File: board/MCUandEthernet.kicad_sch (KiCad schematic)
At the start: 3 parts, among them J1 RJ45_LED_Shielded, U15 Teensy4.1_DEV-16771

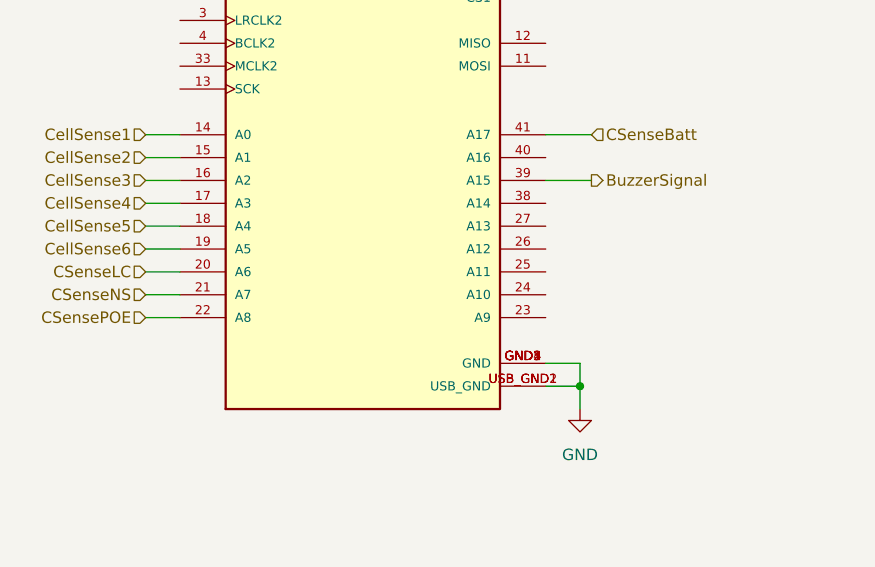
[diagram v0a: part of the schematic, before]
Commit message: Replaced Current sensors and made aux current sensor
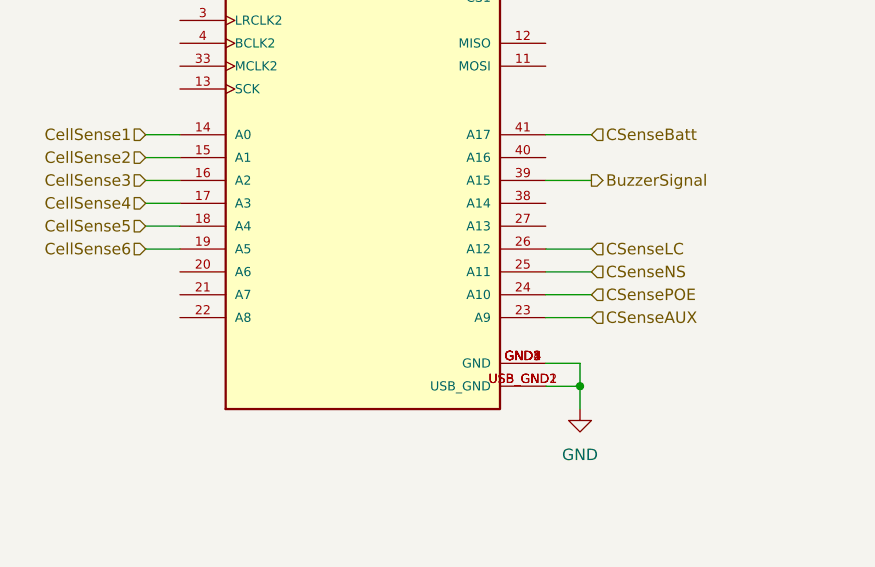
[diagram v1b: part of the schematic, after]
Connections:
- net CSenseLC: now also U15.26 (A12); no longer U15.20 (A6)
- net CSenseNS: now also U15.25 (A11); no longer U15.21 (A7)
- net CSensePOE: now also U15.24 (A10); no longer U15.22 (A8)
- net CSenseAUX: now reaches U15.23 (A9)
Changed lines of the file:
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@@
-	(wire
-		(pts
-			(xy 24.13 134.62) (xy 27.94 134.62)
-		)
-		(stroke
-			(width 0)
-			(type default)
-		)
-	)
 	(wire
 		(pts
@@
 	(wire
 		(pts
+			(xy 68.58 127) (xy 73.66 127)
+		)
+		(stroke
+			(width 0)
+			(type default)
+		)
+	)
+	(wire
+		(pts
 			(xy 142.24 160.02) (xy 142.24 152.4)
 		)
@@
 	(wire
 		(pts
-			(xy 24.13 129.54) (xy 27.94 129.54)
-		)
-		(stroke
-			(width 0)
-			(type default)
-		)
-	)
-	(wire
-		(pts
 			(xy 73.66 69.85) (xy 71.12 69.85)
 		)
@@
 	(wire
 		(pts
-			(xy 24.13 132.08) (xy 27.94 132.08)
+			(xy 68.58 134.62) (xy 73.66 134.62)
 		)
 		(stroke
@@
 	(wire
 		(pts
+			(xy 68.58 132.08) (xy 73.66 132.08)
+		)
+		(stroke
+			(width 0)
+			(type default)
+		)
+	)
+	(wire
+		(pts
 			(xy 128.27 138.43) (xy 128.27 162.56)
+		)
+		(stroke
+			(width 0)
+			(type default)
+		)
+	)
+	(wire
+		(pts
+			(xy 68.58 129.54) (xy 73.66 129.54)
 		)
 		(stroke
@@
 	(hierarchical_label "CSensePOE"
 		(shape input)
-		(at 24.13 134.62 180)
-		(effects
-			(font
-				(size 1.27 1.27)
-			)
-			(justify right)
+		(at 73.66 132.08 0)
+		(effects
+			(font
+				(size 1.27 1.27)
+			)
+			(justify left)
 		)
 	)
@@
 		)
 	)
+	(hierarchical_label "CSenseAUX"
+		(shape input)
+		(at 73.66 134.62 0)
+		(effects
+			(font
+				(size 1.27 1.27)
+			)
+			(justify left)
+		)
+	)
 	(hierarchical_label "CSenseLC"
 		(shape input)
-		(at 24.13 129.54 180)
-		(effects
-			(font
-				(size 1.27 1.27)
-			)
-			(justify right)
+		(at 73.66 127 0)
+		(effects
+			(font
+				(size 1.27 1.27)
+			)
+			(justify left)
 		)
 	)
 	(hierarchical_label "CSenseNS"
 		(shape input)
-		(at 24.13 132.08 180)
-		(effects
-			(font
-				(size 1.27 1.27)
-			)
-			(justify right)
-		)
-	)
+		(at 73.66 129.54 0)
+		(effects
+			(font
+				(size 1.27 1.27)
+			)
+			(justify left)
+		)
+	)

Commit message: Revert "Replaced Current sensors and made aux current sensor"
This reverts commit 6ac851d0f9d66083f206abad37eab70415909eb9.
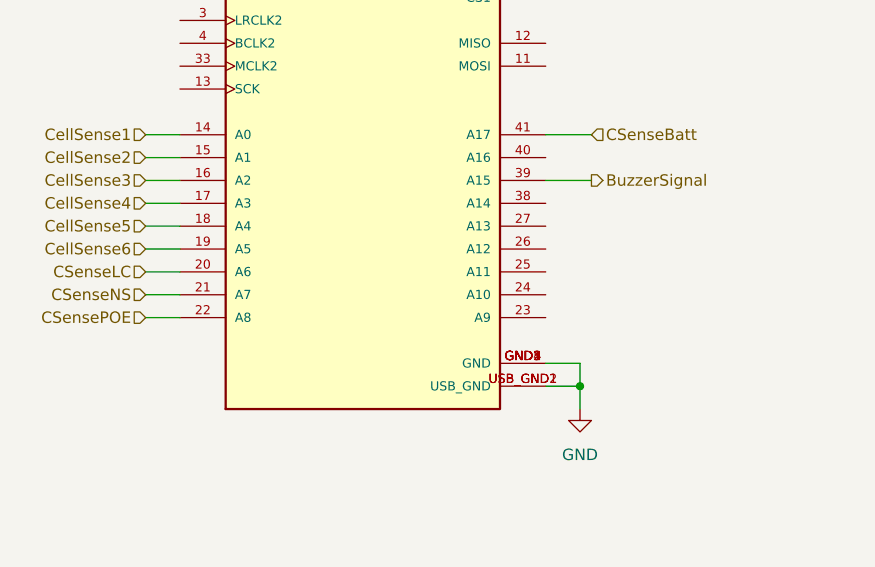
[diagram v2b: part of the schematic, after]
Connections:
- net CSenseLC: now also U15.20 (A6); no longer U15.26 (A12)
- net CSenseNS: now also U15.21 (A7); no longer U15.25 (A11)
- net CSensePOE: now also U15.22 (A8); no longer U15.24 (A10)
- net CSenseAUX: no longer names the net of U15.23 (A9)
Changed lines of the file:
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@@
+	(wire
+		(pts
+			(xy 24.13 134.62) (xy 27.94 134.62)
+		)
+		(stroke
+			(width 0)
+			(type default)
+		)
+	)
 	(wire
 		(pts
@@
 	(wire
 		(pts
-			(xy 68.58 127) (xy 73.66 127)
-		)
-		(stroke
-			(width 0)
-			(type default)
-		)
-	)
-	(wire
-		(pts
 			(xy 142.24 160.02) (xy 142.24 152.4)
 		)
@@
 	(wire
 		(pts
+			(xy 24.13 129.54) (xy 27.94 129.54)
+		)
+		(stroke
+			(width 0)
+			(type default)
+		)
+	)
+	(wire
+		(pts
 			(xy 73.66 69.85) (xy 71.12 69.85)
 		)
@@
 	(wire
 		(pts
-			(xy 68.58 134.62) (xy 73.66 134.62)
+			(xy 24.13 132.08) (xy 27.94 132.08)
 		)
 		(stroke
@@
 	(wire
 		(pts
-			(xy 68.58 132.08) (xy 73.66 132.08)
-		)
-		(stroke
-			(width 0)
-			(type default)
-		)
-	)
-	(wire
-		(pts
 			(xy 128.27 138.43) (xy 128.27 162.56)
-		)
-		(stroke
-			(width 0)
-			(type default)
-		)
-	)
-	(wire
-		(pts
-			(xy 68.58 129.54) (xy 73.66 129.54)
 		)
 		(stroke
@@
 	(hierarchical_label "CSensePOE"
 		(shape input)
-		(at 73.66 132.08 0)
-		(effects
-			(font
-				(size 1.27 1.27)
-			)
-			(justify left)
+		(at 24.13 134.62 180)
+		(effects
+			(font
+				(size 1.27 1.27)
+			)
+			(justify right)
 		)
 	)
@@
 		)
 	)
-	(hierarchical_label "CSenseAUX"
-		(shape input)
-		(at 73.66 134.62 0)
-		(effects
-			(font
-				(size 1.27 1.27)
-			)
-			(justify left)
-		)
-	)
 	(hierarchical_label "CSenseLC"
 		(shape input)
-		(at 73.66 127 0)
-		(effects
-			(font
-				(size 1.27 1.27)
-			)
-			(justify left)
+		(at 24.13 129.54 180)
+		(effects
+			(font
+				(size 1.27 1.27)
+			)
+			(justify right)
 		)
 	)
 	(hierarchical_label "CSenseNS"
 		(shape input)
-		(at 73.66 129.54 0)
-		(effects
-			(font
-				(size 1.27 1.27)
-			)
-			(justify left)
-		)
-	)
+		(at 24.13 132.08 180)
+		(effects
+			(font
+				(size 1.27 1.27)
+			)
+			(justify right)
+		)
+	)
